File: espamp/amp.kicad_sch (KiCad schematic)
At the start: 1 part, among them U501 TAS5825MRHB

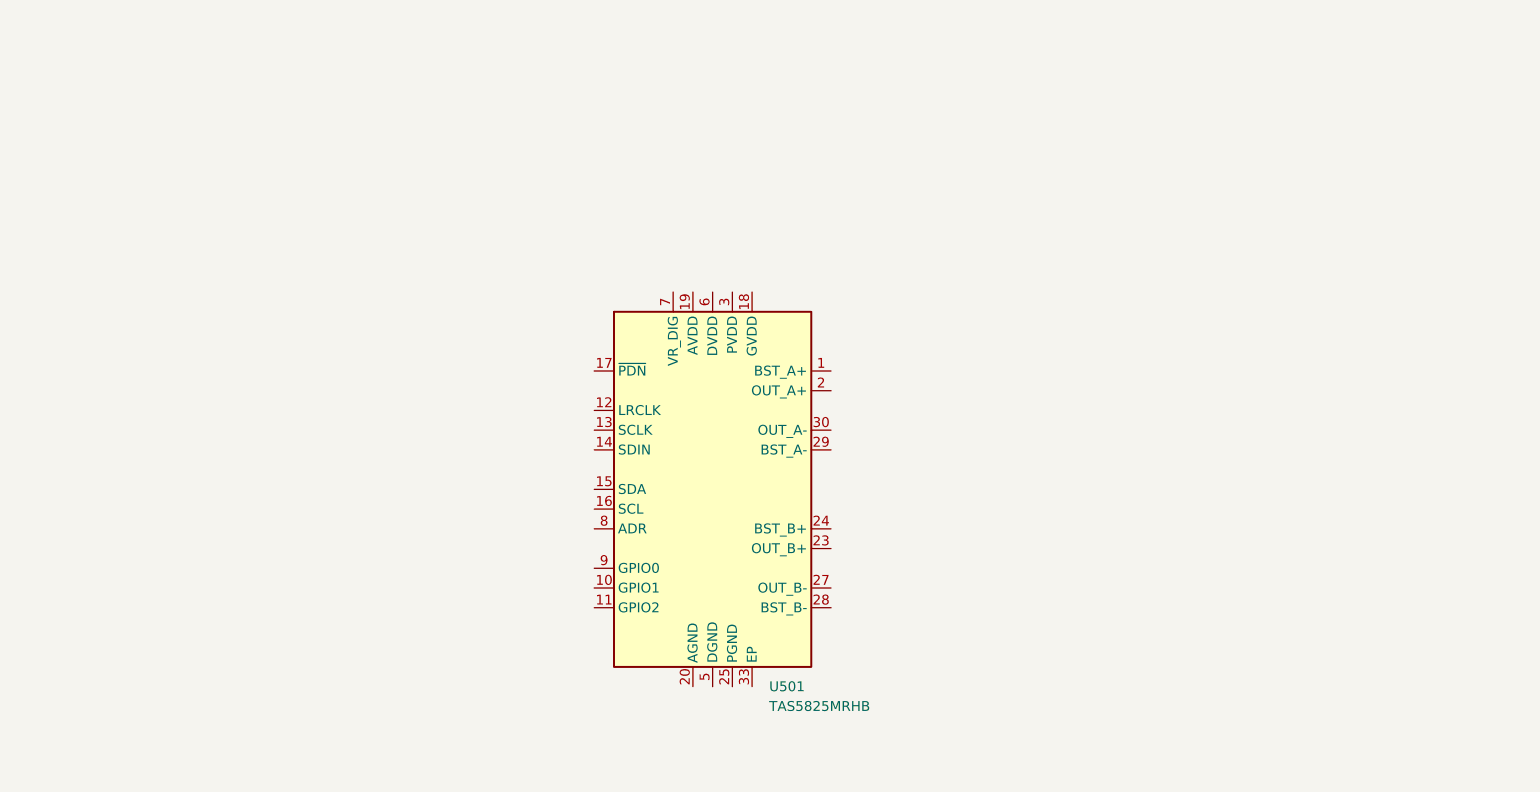
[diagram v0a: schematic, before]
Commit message: amp schematic draft
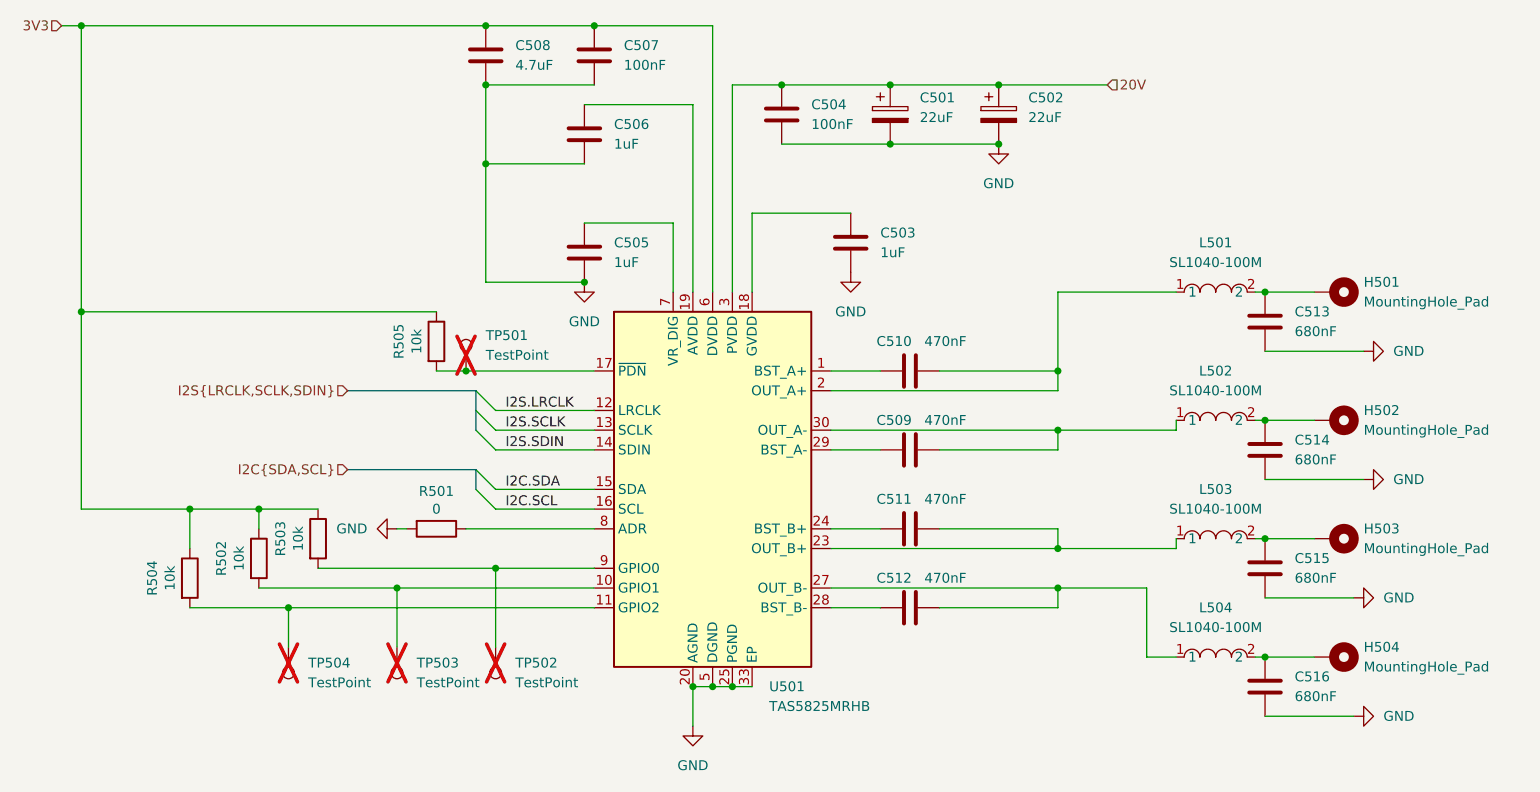
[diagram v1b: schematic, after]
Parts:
- added C501, C502: 22uF, Capacitor_SMD:C_Elec_5x5.8, symbol Device:C_Polarized
- added C503, C505, C506: 1uF, Capacitor_SMD:C_0603_1608Metric, symbol Device:C
- added C504, C507: 100nF, Capacitor_SMD:C_0603_1608Metric, symbol Device:C
- added C508: 4.7uF, Capacitor_SMD:C_0603_1608Metric, symbol Device:C
- added C509, C510, C511, C512: 470nF, Capacitor_SMD:C_0603_1608Metric, symbol Device:C
- added C513, C514, C515, C516: 680nF, Capacitor_SMD:C_0603_1608Metric, symbol Device:C
- added H501, H502, H503, H504: MountingHole_Pad, MountingHole:MountingHole_4mm_Pad_Via, symbol Mechanical:MountingHole_Pad
- added L501, L502, L503, L504: SL1040-100M, easyeda2kicad:IND-SMD_L11.0-W10.2, symbol easyeda2kicad:SL1040-100M
- added R501: 0, Resistor_SMD:R_0603_1608Metric, symbol Device:R
- added R502, R503, R504, R505: 10k, Resistor_SMD:R_0603_1608Metric, symbol Device:R
- added TP501, TP502, TP503, TP504: TestPoint, Connector_PinHeader_1.00mm:PinHeader_1x01_P1.00mm_Vertical, symbol Connector:TestPoint
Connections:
- net at U501.1 (BST_A+): now also C510.1
- net at U501.10 (GPIO1): now also R502.2, TP503.1
- net at U501.11 (GPIO2): now also R504.2, TP504.1
- net I2S.LRCLK: now reaches U501.12 (LRCLK)
- net I2S.SCLK: now reaches U501.13 (SCLK)
- net I2S.SDIN: now reaches U501.14 (SDIN)
- net I2C.SDA: now reaches U501.15 (SDA)
- net I2C.SCL: now reaches U501.16 (SCL)
- net at U501.17 (~{PDN}): now also R505.2, TP501.1
- net at U501.18 (GVDD): now also C503.1
- net at U501.19 (AVDD): now also C506.1
- net at U501.2 (OUT_A+): now also C510.2, L501.1
- net GND: now reaches U501.20 (AGND)
- net GND: now also U501.25 (PGND), U501.26 (PGND), U501.31 (PGND), U501.32 (PGND), U501.33 (EP), U501.5 (DGND), C501.2, C502.2, C503.2, C504.2, C505.2, C506.2, C507.2, C508.2, C513.2, C514.2, C515.2, C516.2, R501.2
- net 20V: now reaches U501.21 (PVDD), U501.22 (PVDD), U501.3 (PVDD), U501.4 (PVDD)
- net 20V: now also C501.1, C502.1, C504.1
- net at U501.23 (OUT_B+): now also C511.2, L503.1
- net at U501.24 (BST_B+): now also C511.1
- net at U501.27 (OUT_B-): now also C512.2, L504.1
- net at U501.28 (BST_B-): now also C512.1
- net at U501.29 (BST_A-): now also C509.1
- net at U501.30 (OUT_A-): now also C509.2, L502.1
- net 3V3: now reaches U501.6 (DVDD)
- net 3V3: now also C507.1, C508.1, R502.1, R503.1, R504.1, R505.1
- net at U501.7 (VR_DIG): now also C505.1
- net at U501.8 (ADR): now also R501.1
- net at U501.9 (GPIO0): now also R503.2, TP502.1
- new net: C516.1, H504.1, L504.2
- new net: C513.1, H501.1, L501.2
- new net: C514.1, H502.1, L502.2
- new net: C515.1, H503.1, L503.2
